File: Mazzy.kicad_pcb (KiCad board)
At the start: 2 copper layers, 100 x 80 mm, 100 parts, among them J1 Conn_01x02_Pin, J10 RJ45_Hanrun_HR911105A_Horizon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, J11 Micro_SD_Card_Det1, J2 Conn_01x02_Pin, J3 USB_C_Receptacle_USB2.0_16P, J4 USB_C_Receptacle_USB2.0_16P, J5 Conn_01x02_Pin, J6 Conn_01x02_Pin, J7 Conn_01x02_Pin, J8 OBD-II, J9 SWC, Q1 DMG2301L, SW1 SW_Push, U1 TPS54302, U10 DS3231MZ, U2 MCP73831-2-OT, U3 MCP100-300D, U4 ESP32-S3-WROOM-1, U5 RP2040, U6 W25Q16JVSS, U7 SN65HVD230, U8 SN65HVD230, U9 W5500, Y1 25MHz

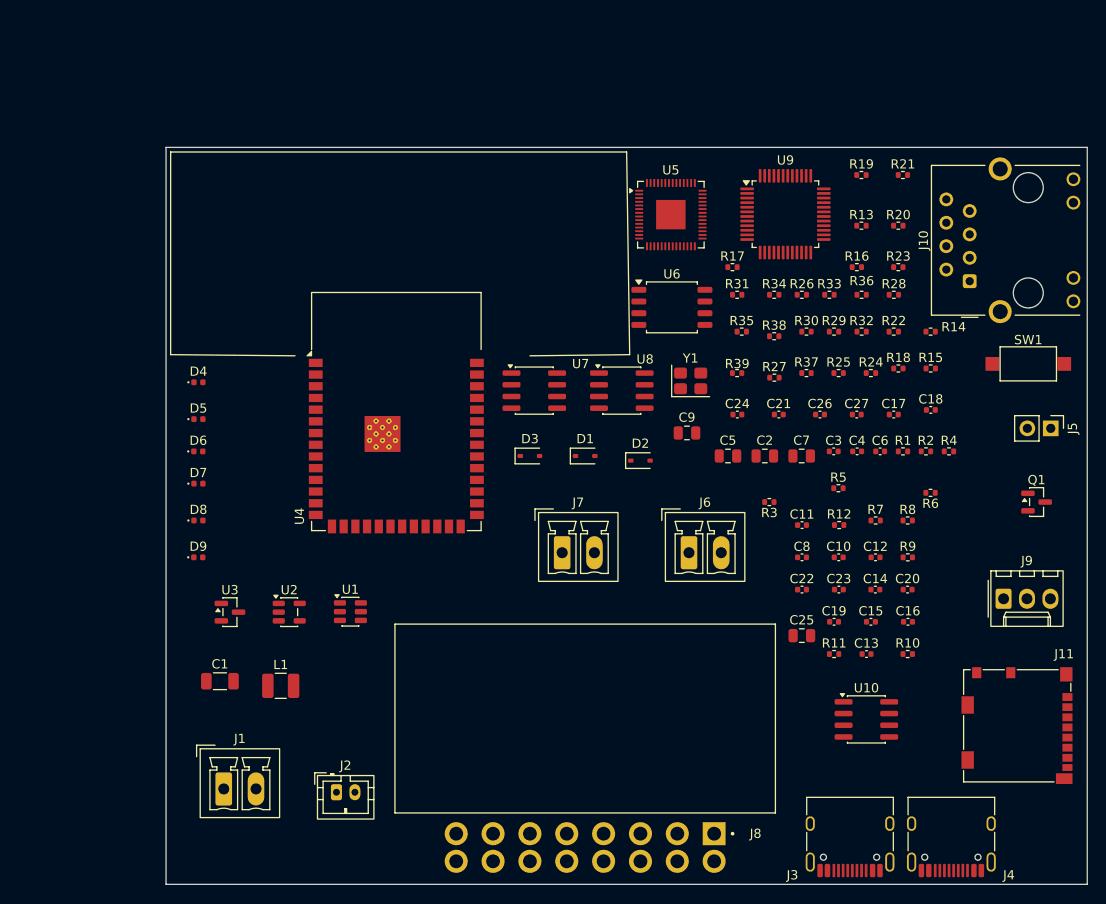
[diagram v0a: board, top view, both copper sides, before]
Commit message: wip
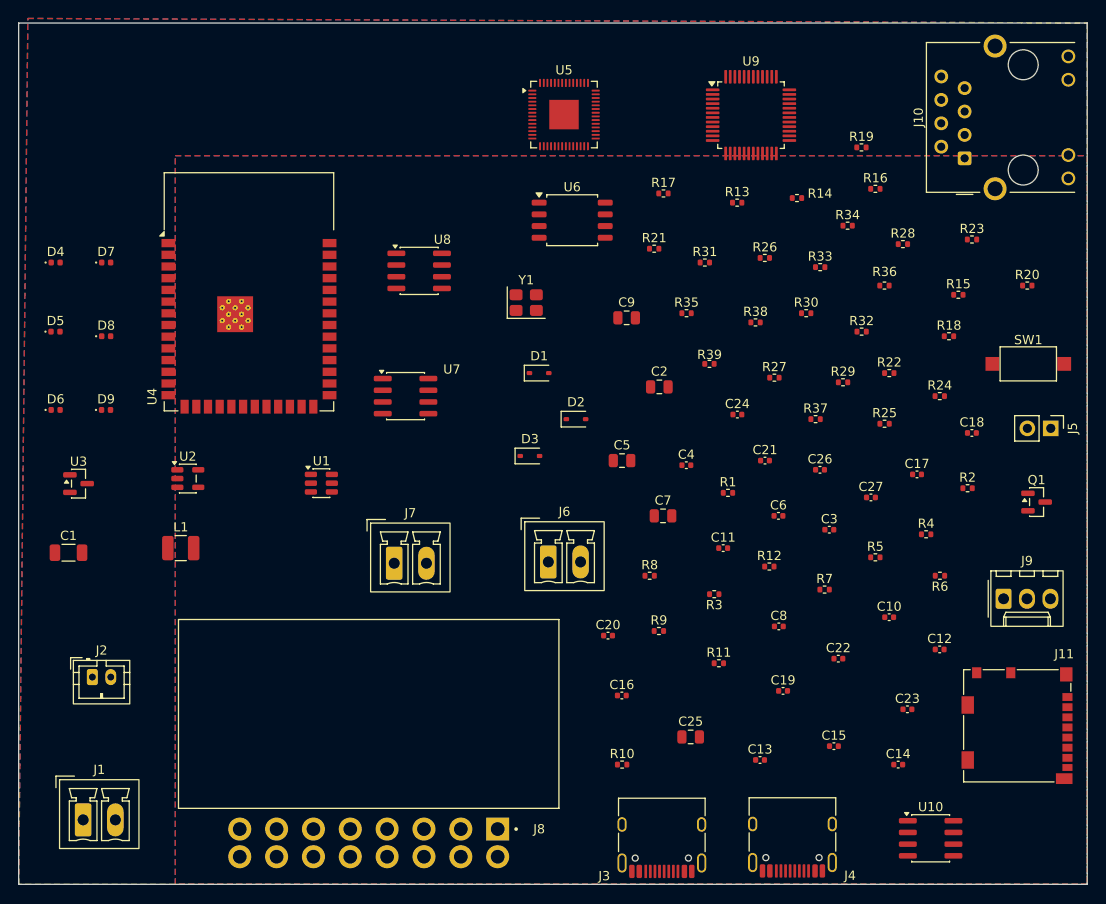
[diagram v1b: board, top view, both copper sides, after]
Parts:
- moved R10 33.2 mm to (188.0, 127.0)
- moved C20 32.9 mm to (186.5, 113.0)
- moved C16 32.1 mm to (188.0, 119.5)
- moved J2 29.3 mm to (130.5, 117.5)
- moved R8 28.6 mm to (191.0, 106.5)
- moved R9 28.2 mm to (192.0, 112.5)
- moved R21 28.2 mm to (191.5, 71.0)
- moved D7 26.0 mm to (132.0, 72.5)
- moved U8 25.6 mm to (166.0, 73.4)
- moved J8 23.5 mm to (174.5, 134.0)
- moved D8 22.4 mm to (132.0, 80.5)
- moved C1 21.6 mm to (127.9, 104.0)
- moved U3 21.6 mm to (129.0, 96.5)
- moved U4 20.6 mm to (147.5, 75.7)
- moved R14 20.5 mm to (207.0, 65.5)
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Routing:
- added copper zone on B.Cu, net GND
- added copper zone on F.Cu, net GND
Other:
- board size 100 x 80 mm -> 116 x 93.5 mm
